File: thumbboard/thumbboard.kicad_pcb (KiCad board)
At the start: 2 copper layers, 63 x 36 mm, 8 parts, among them J1 Conn_01x05_MountingPin, SW1 SW_Push, SW2 SW_Push, SW3 SW_Push, SW4 SW_Push

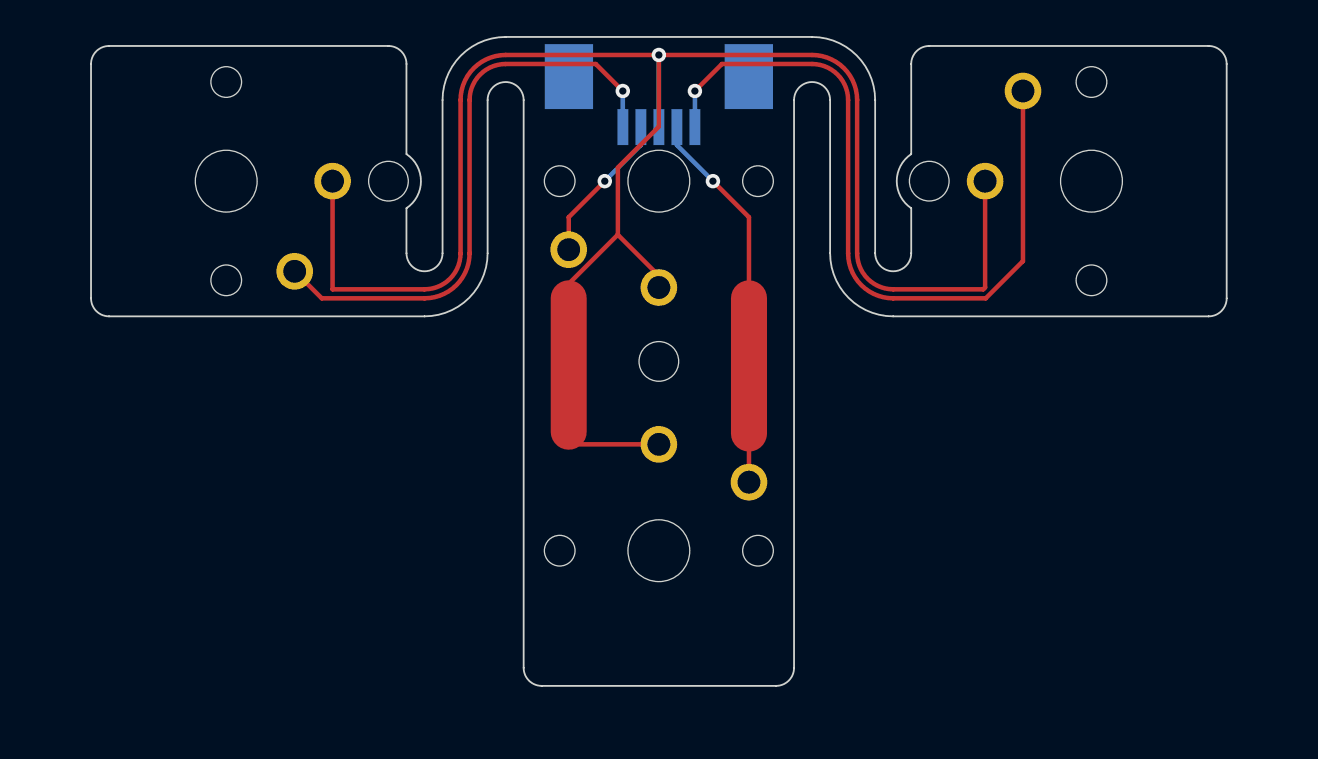
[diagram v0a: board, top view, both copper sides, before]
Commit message: various tweaks, about to start on the carapace
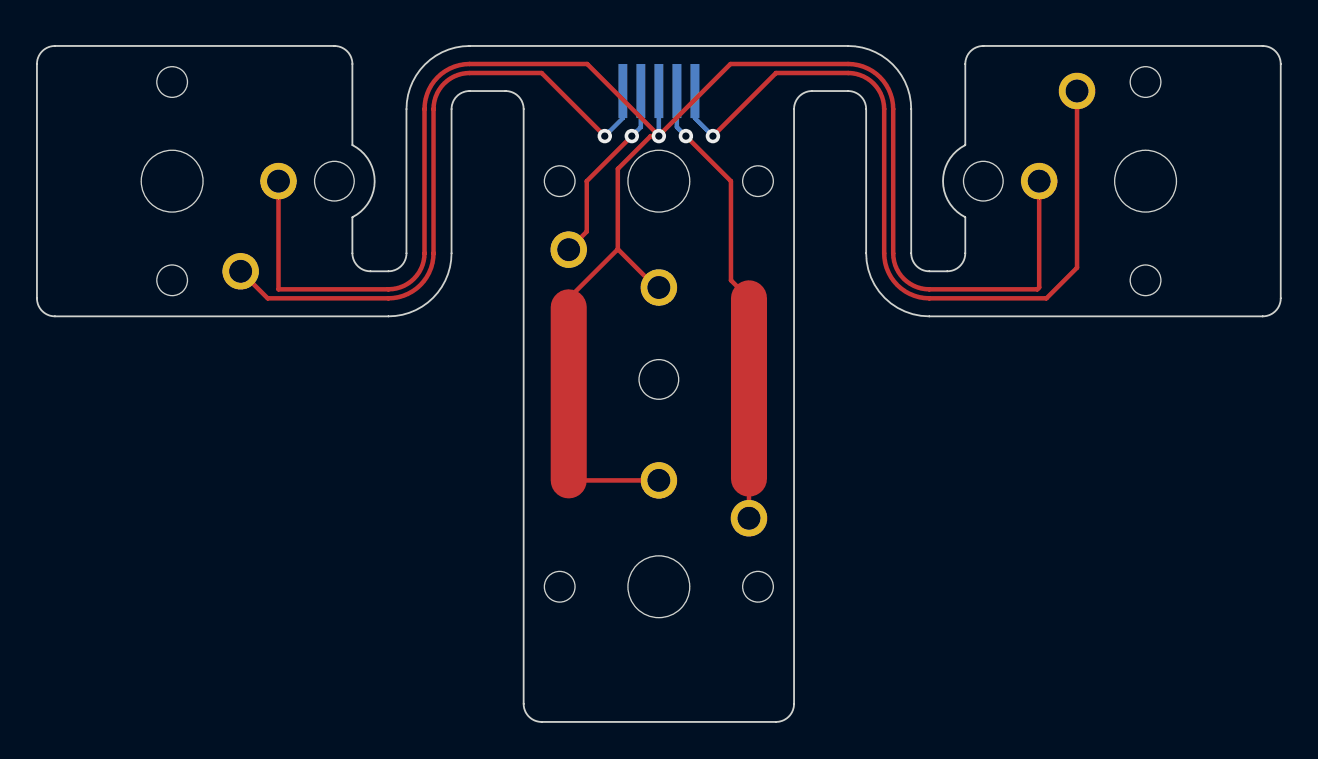
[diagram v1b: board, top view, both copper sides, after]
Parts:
- added T1: Tab, PCM_kikit:Tab, F.Cu at (118.0, 77.2)
- added T2: Tab, PCM_kikit:Tab, F.Cu at (110.2, 85.0)
- added T3: Tab, PCM_kikit:Tab, F.Cu at (145.0, 77.2)
- added T4: Tab, PCM_kikit:Tab, F.Cu at (172.0, 77.2)
- added T5: Tab, PCM_kikit:Tab, F.Cu at (179.8, 85.0)
- added T6: Tab, PCM_kikit:Tab, F.Cu at (145.0, 115.2)
- J1: footprint Connector_FFC-FPC:TE_84952-5_1x05-1MP_P1.0mm_Horizontal -> panelization:FFC clamp fit 1x05 1.00mm
- moved REF** 3.00 mm to (127.0, 85.0)
- moved REF** 3.00 mm to (163.0, 85.0)
- moved SW1 3.00 mm to (118.0, 85.0)
- moved SW4 3.00 mm to (172.0, 85.0)
- moved SW3 2.00 mm to (145.0, 107.5)
- moved REF** 1.00 mm to (145.0, 96.0)
- moved J1 0.20 mm to (145.0, 80.0), turned to 180 degrees
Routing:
- net COL: track 104.6 -> 110.4 mm
- net ROW_C: track 20.9 -> 25.4 mm
- net ROW_D: track 42.0 -> 45.5 mm
- net ROW_A: track 32.3 -> 35.6 mm
- net ROW_B: track 8.46 -> 10.5 mm
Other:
- board size 63 x 36 mm -> 69 x 37.5 mm
